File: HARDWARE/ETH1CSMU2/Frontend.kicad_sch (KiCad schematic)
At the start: 60 parts, among them Q601 MMBT3904, Q602 MMBT3904, Q603 MMBT3904, U601 DG419DY, U602 DG419DY, U603 SN74LVC1T45DRLR, U604 SN74LVC1T45DRLR, U605 SN74LVC1T45DRLR, U606 LT1970ACFE, U607 AQY212G2SX, U608 AQY212G2SX, U609 AQY212G2SX, U610 INA823DT

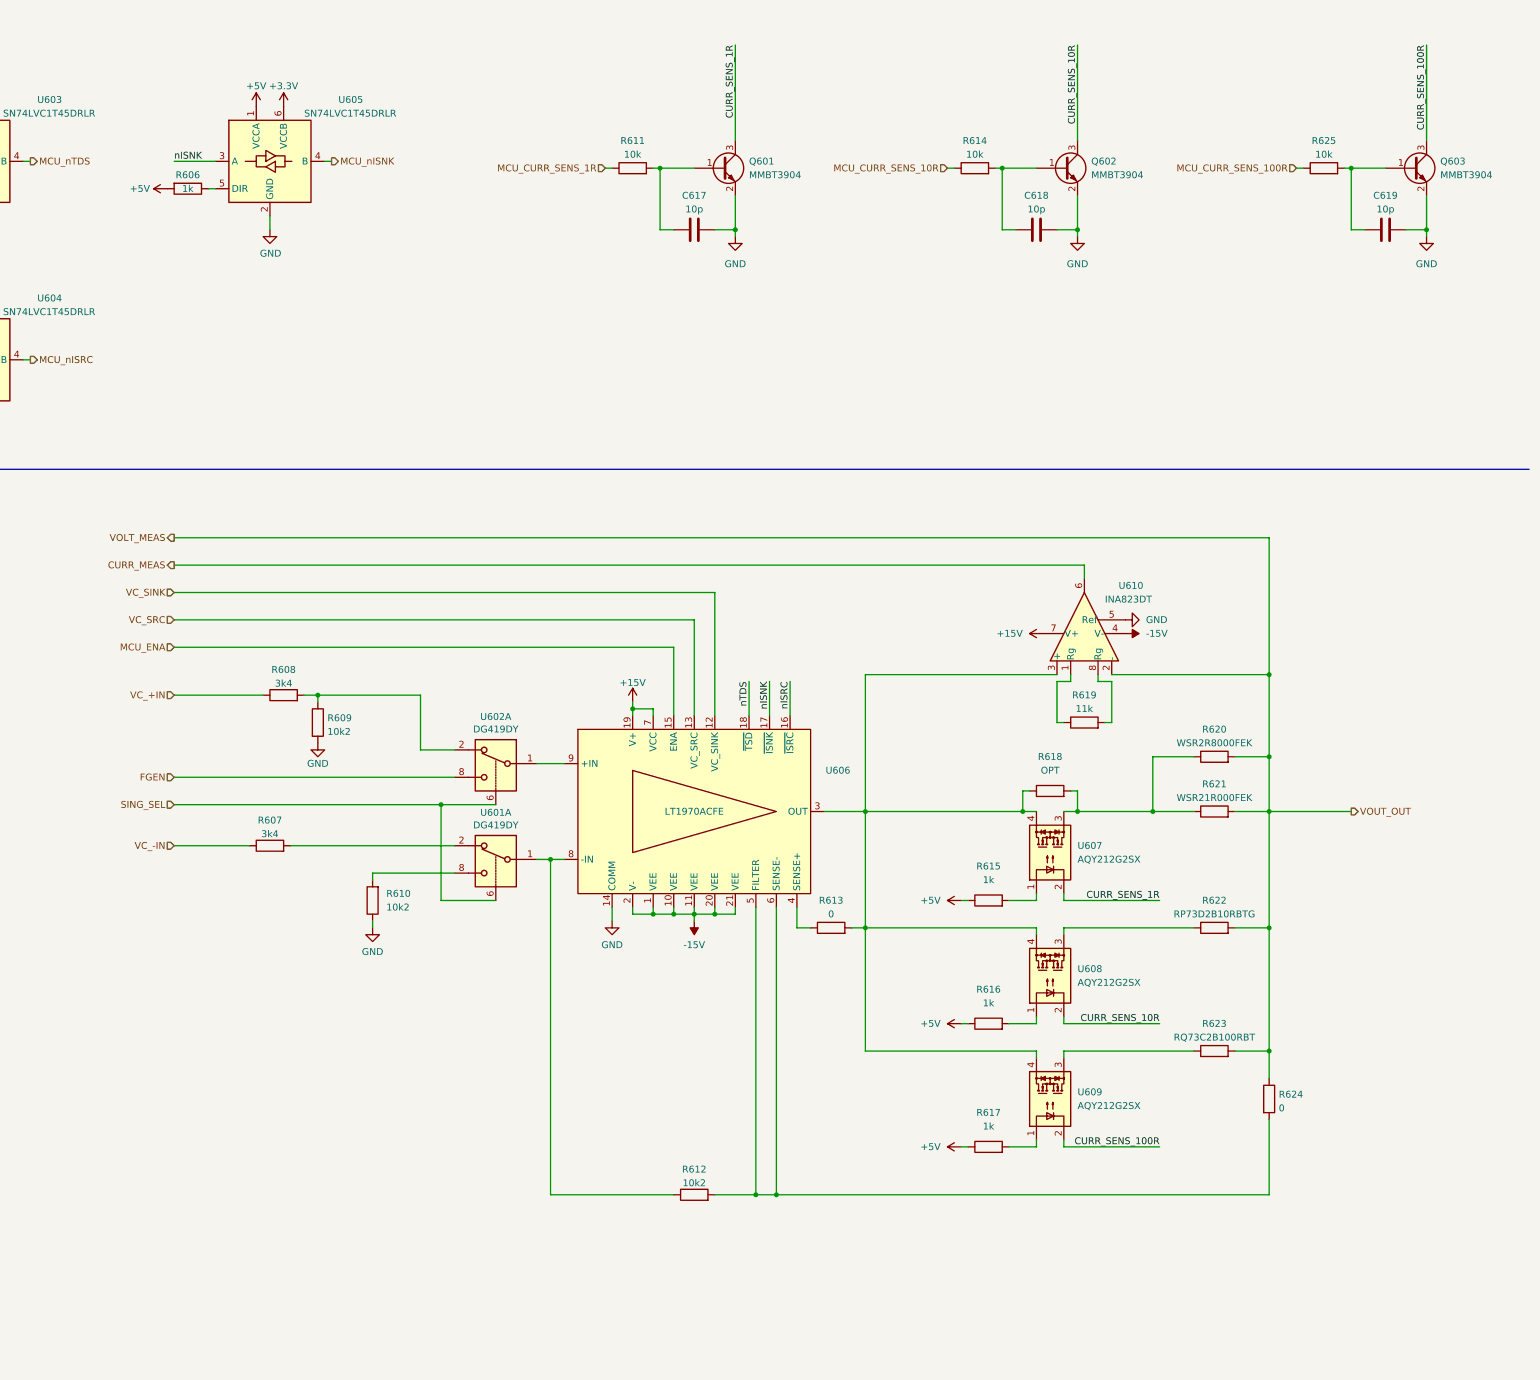
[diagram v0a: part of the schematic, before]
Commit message: Hardware design
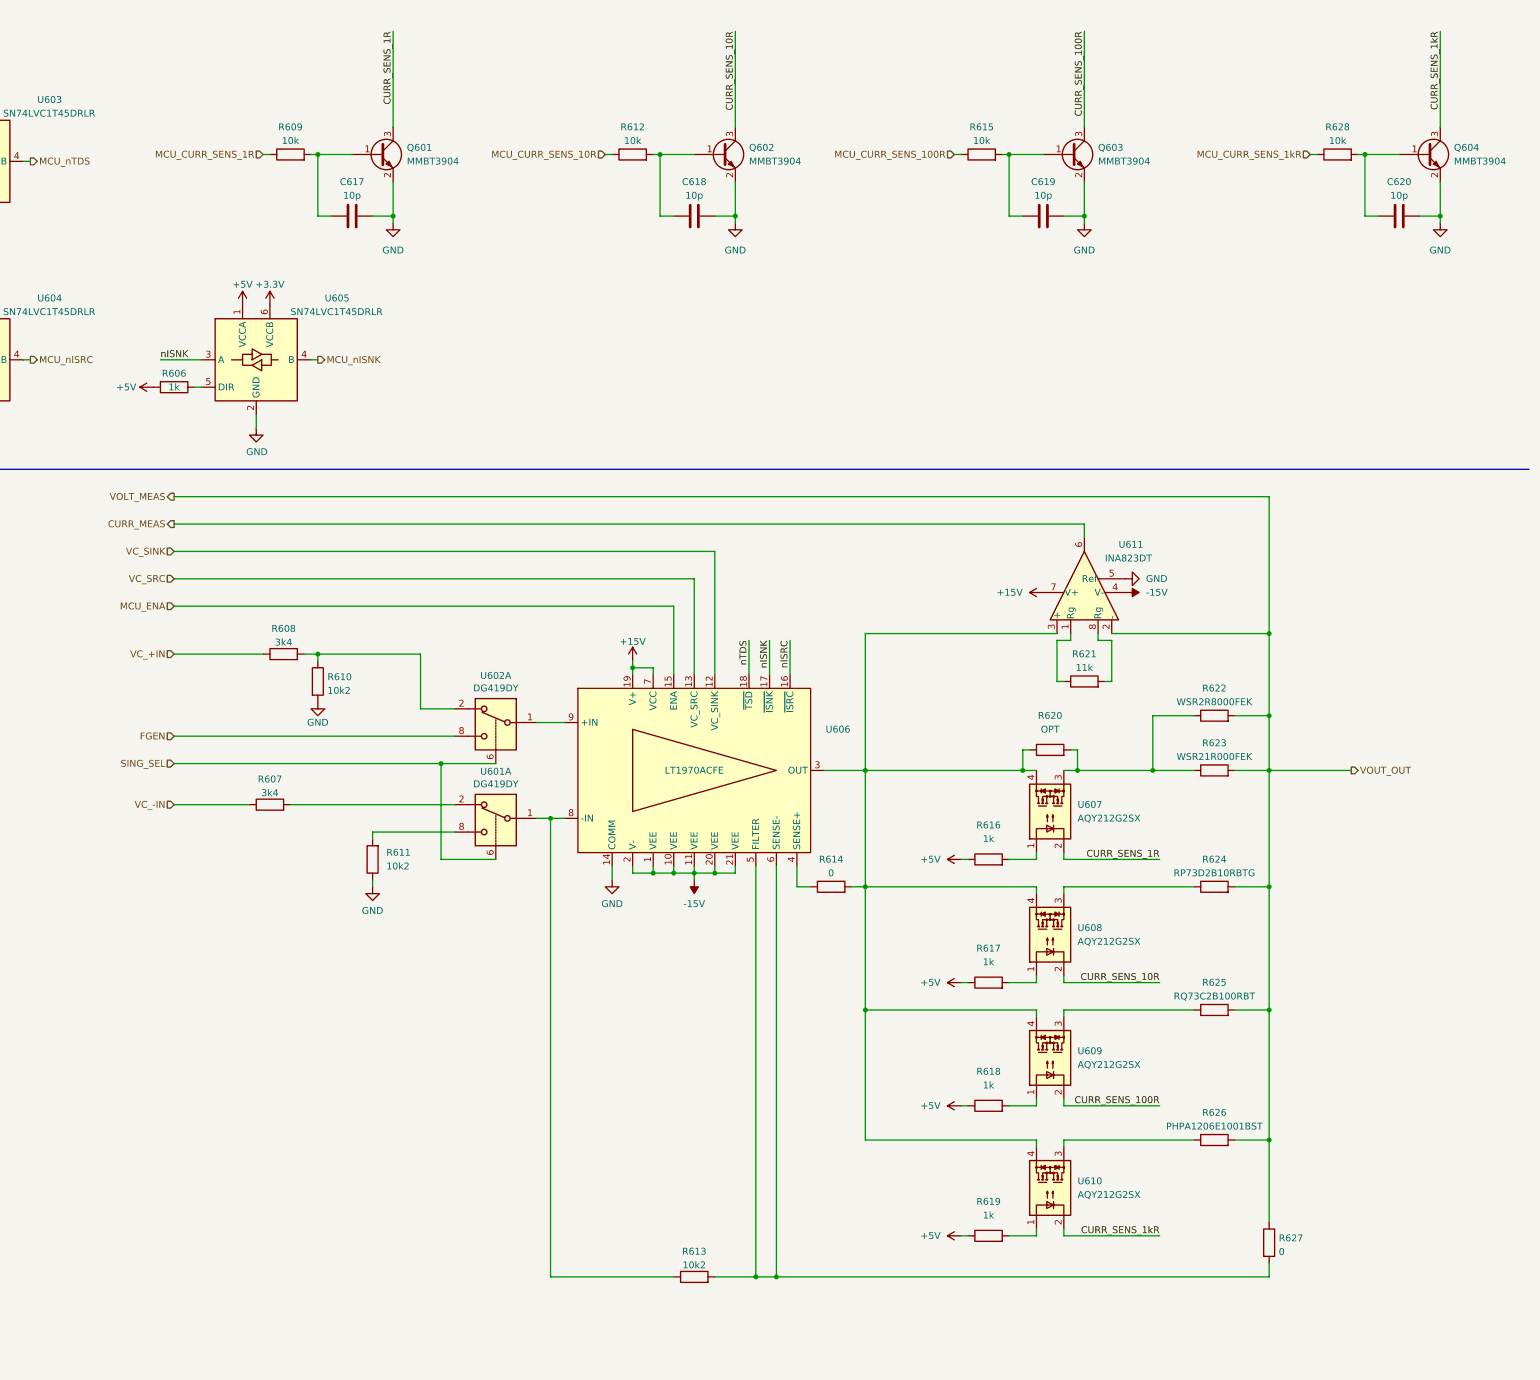
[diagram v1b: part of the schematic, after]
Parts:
- added C620: 10p, Capacitor_SMD:C_0603_1608Metric_Pad1.08x0.95mm_HandSolder, symbol Device:C
- added Q604: MMBT3904, Package_TO_SOT_SMD:SOT-23, symbol Transistor_BJT:MMBT3904
- added R619: 1k, Resistor_SMD:R_0603_1608Metric_Pad0.98x0.95mm_HandSolder, symbol Device:R
- added R626: PHPA1206E1001BST, Resistor_SMD:R_1206_3216Metric_Pad1.30x1.75mm_HandSolder, symbol Device:R
- added R628: 10k, Resistor_SMD:R_0603_1608Metric_Pad0.98x0.95mm_HandSolder, symbol Device:R
- added U610: AQY212G2SX, ETH1CSMU2:AQY212GS, symbol ETH1CSMU2:AQY212GS
- renumbered R611 to R609, R609 to R610, R610 to R611, R614 to R612, R612 to R613, R613 to R614, R625 to R615, R615 to R616, R616 to R617, R617 to R618, R618 to R620, R619 to R621, R620 to R622, R621 to R623, R622 to R624, R623 to R625, R624 to R627, U610 to U611
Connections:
- net +5V: now also R619.1
- net GND: now also C620.2, Q604.2 (E)
- net VOLT_MEAS: now also R626.2
- net at R614.2, R620.1, U606.3 (OUT)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: now also U610.4
- new net: C620.1, Q604.1 (B), R628.2
- new net: R619.2, U610.1
- new net: R626.1, U610.3
- new net CURR_SENS_1kR: Q604.3 (C), U610.2
- new net MCU_CURR_SENS_1kR: R628.1
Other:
- moved on the sheet: C617, C618, C619, Q601, Q602, Q603, R606, R607, R608, R609, R610, R611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
